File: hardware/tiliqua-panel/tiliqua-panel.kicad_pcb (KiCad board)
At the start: 2 copper layers, 30 x 128.5 mm, 13 parts

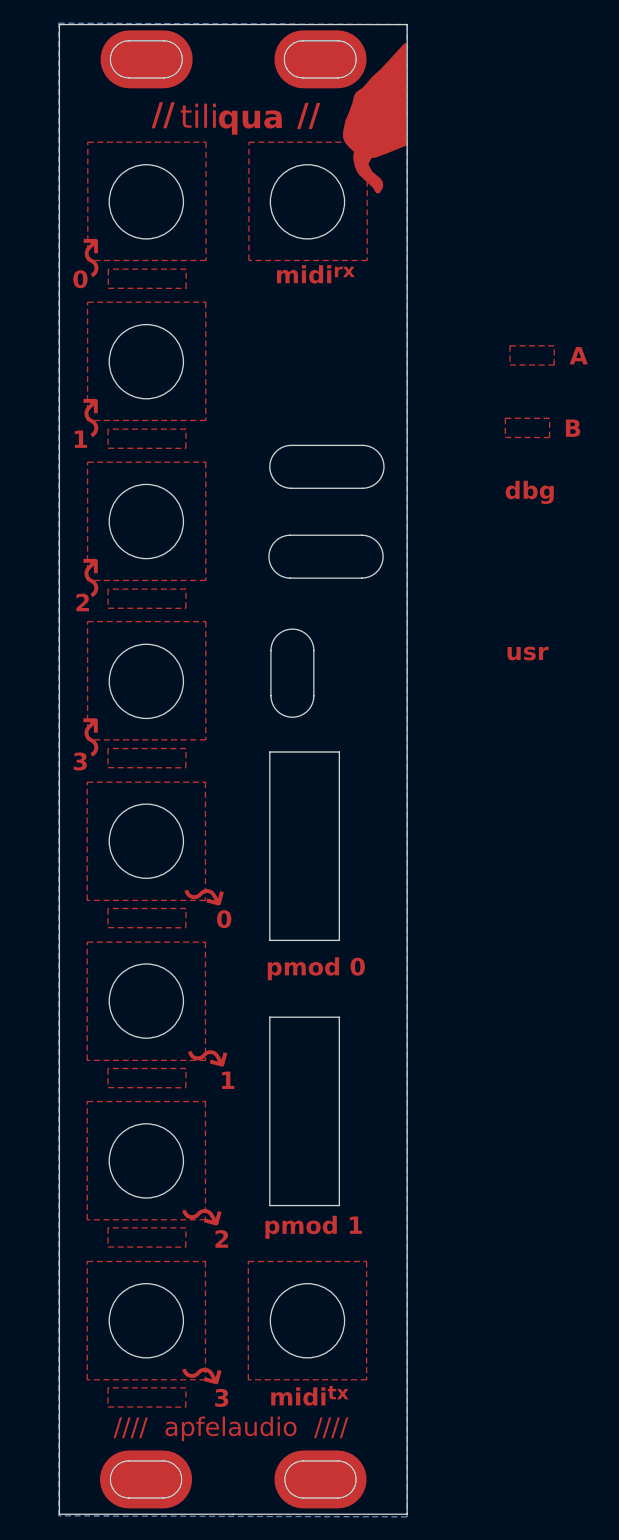
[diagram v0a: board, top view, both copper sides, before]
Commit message: after panel swap
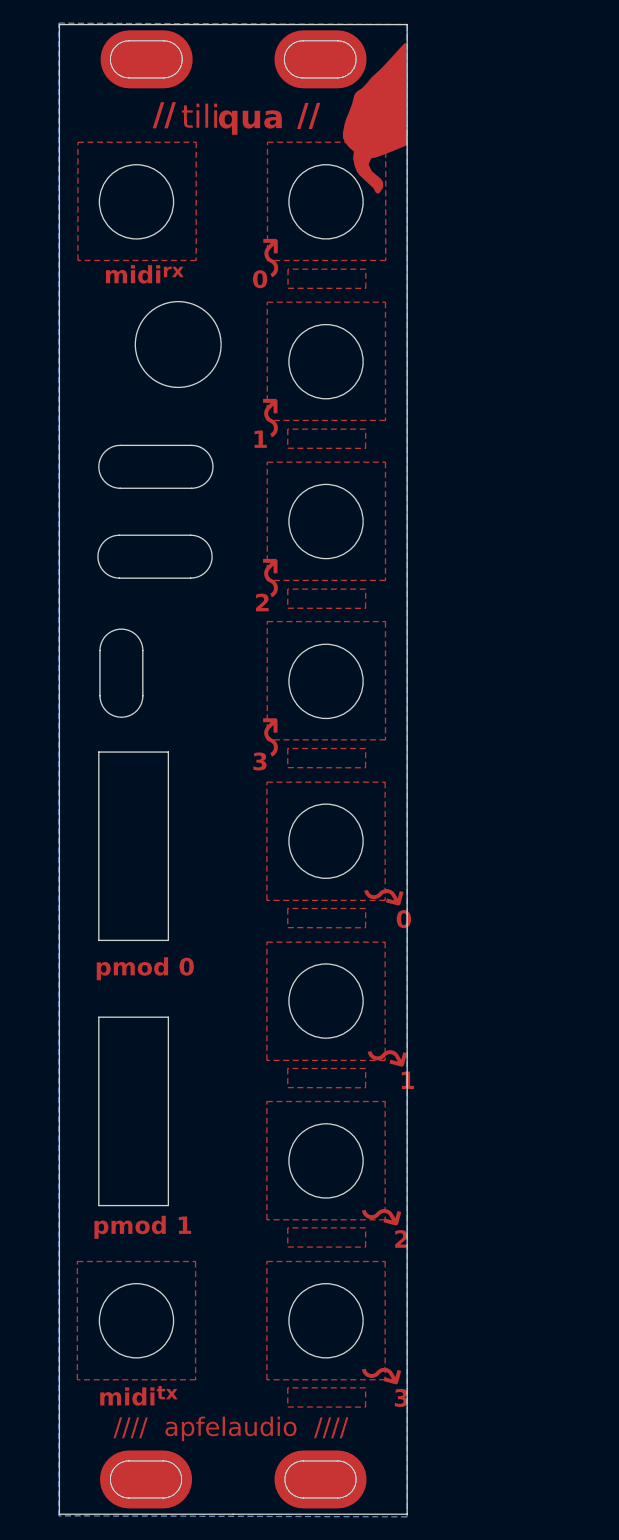
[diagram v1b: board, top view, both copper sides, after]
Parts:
- added REF**: MountingHole_7.4mm_M6, MountingHole:MountingHole_6.4mm_M6, F.Cu at (7.25, 27.6)
- moved REF** 15.5 mm to (20.0, 111.8)
- moved REF** 15.5 mm to (20.0, 70.4)
- moved REF** 15.5 mm to (20.0, 29.1)
- moved REF** 15.5 mm to (20.0, 84.2)
- moved REF** 15.5 mm to (20.0, 42.9)
- moved REF** 15.5 mm to (20.0, 15.3)
- moved REF** 15.5 mm to (20.0, 98.0)
- moved REF** 15.5 mm to (20.0, 56.7)
- moved REF** 14.8 mm to (14.8, 8.65)
- moved REF** 14.8 mm to (-0.85, 9.00)
- moved REF** 14.7 mm to (3.65, 15.3)
- moved REF** 14.7 mm to (3.65, 111.8)
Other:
- outline, holes or cut-outs redrawn
- board text removed: "A"
- board text removed: "B"
- board text removed: "dbg"
- board text removed: "usr"
